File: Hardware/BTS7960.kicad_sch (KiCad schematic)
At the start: 37 parts, among them J10 Screw_Terminal_01x04, J11 Screw_Terminal_01x04, J4 Screw_Terminal_01x04, U7 HCPL-2631, U8 HCPL-2631

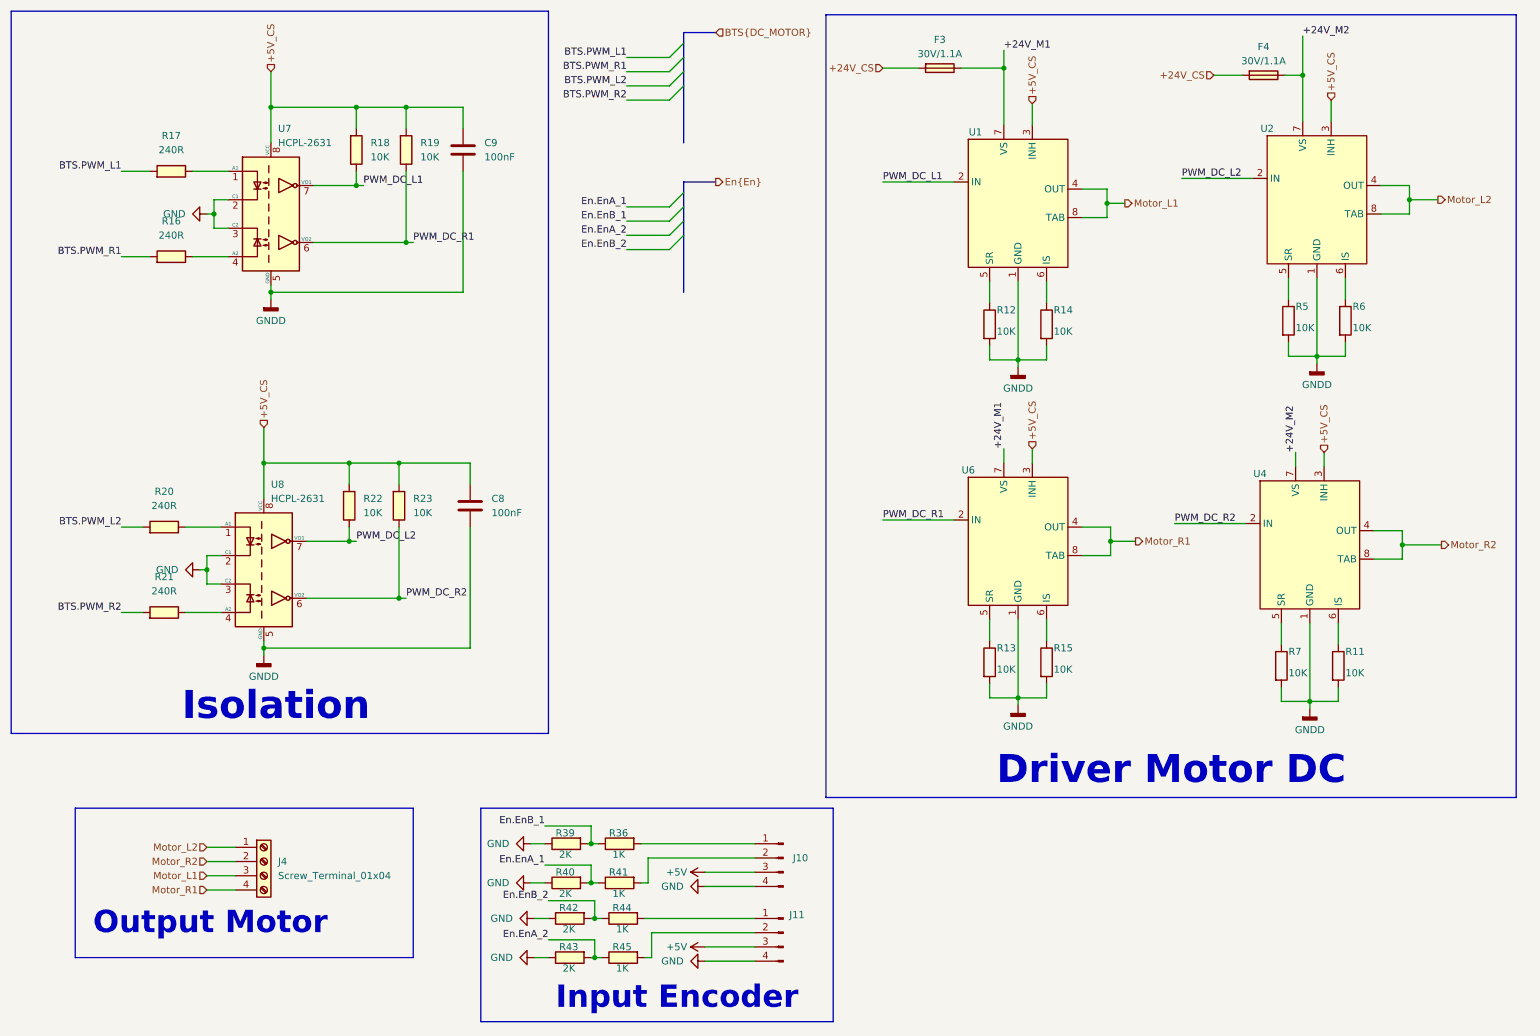
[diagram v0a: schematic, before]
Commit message: Update README
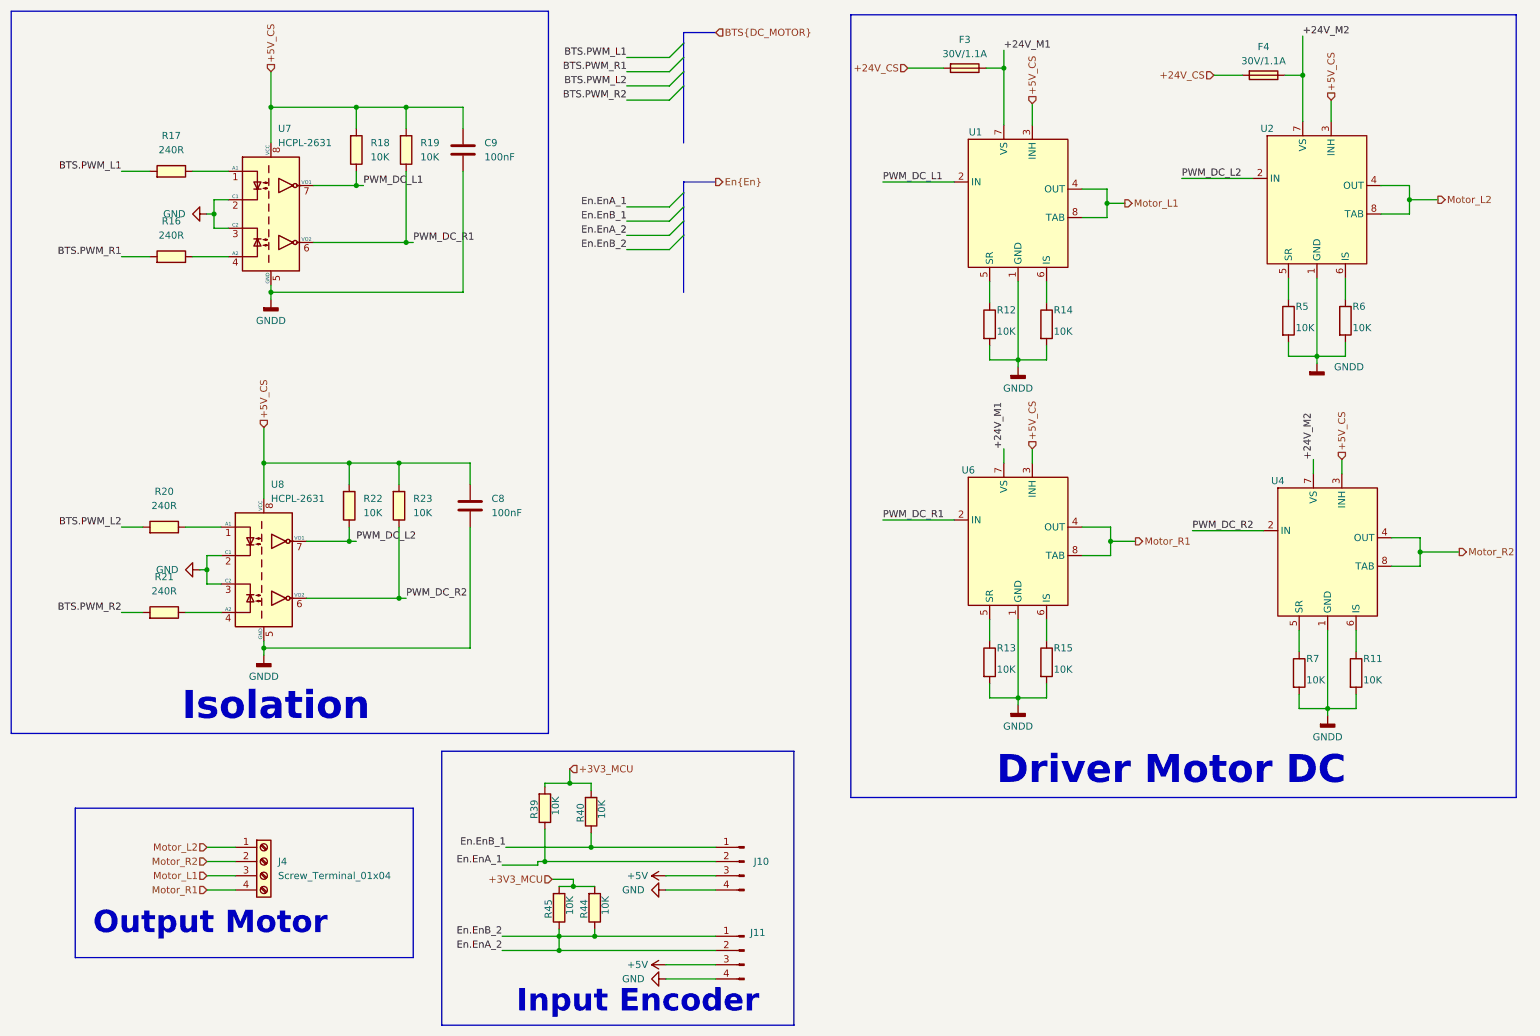
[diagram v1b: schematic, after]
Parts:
- removed R36, R41: 1K, IVS_FOOTPRINTS:R_0603, symbol IVS_SYMBOLS:R
- removed R42, R43: 2K, IVS_FOOTPRINTS:R_0603, symbol IVS_SYMBOLS:R
- R39, R40: value 2K -> 10K
- R44, R45: value 1K -> 10K
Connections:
- net En.EnB_2 is gone; now on net En.EnA_2: R44.2
- net En.EnA_1: now also J10.2 (Pin_2), R39.2; no longer R40.1
- net En.EnA_2: now also J11.1 (Pin_1), J11.2 (Pin_2)
- net En.EnB_1: now also J10.1 (Pin_1), R40.2; no longer R39.1
- net GND: no longer R39.2, R40.2
- net +3V3_MCU: now reaches R44.1
- net +3V3_MCU: now also R39.1, R40.1, R45.1; no longer J11.1 (Pin_1)
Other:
- moved on the sheet: F3, J10, J11, R11, R44, R45, R7, U4
